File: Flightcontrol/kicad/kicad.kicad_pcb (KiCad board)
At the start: 2 copper layers, 55 x 35.1 mm, 53 parts, among them J1 Conn_01x04_Pin, J2 Conn_01x06, J3 Conn_01x08, J4 Conn_01x01_Pin, J5 Conn_01x05, J6 Conn_01x03_Pin, J7 Conn_01x05, U1 ESP32-S3-WROOM-1U-N16R8, U2 BMP581

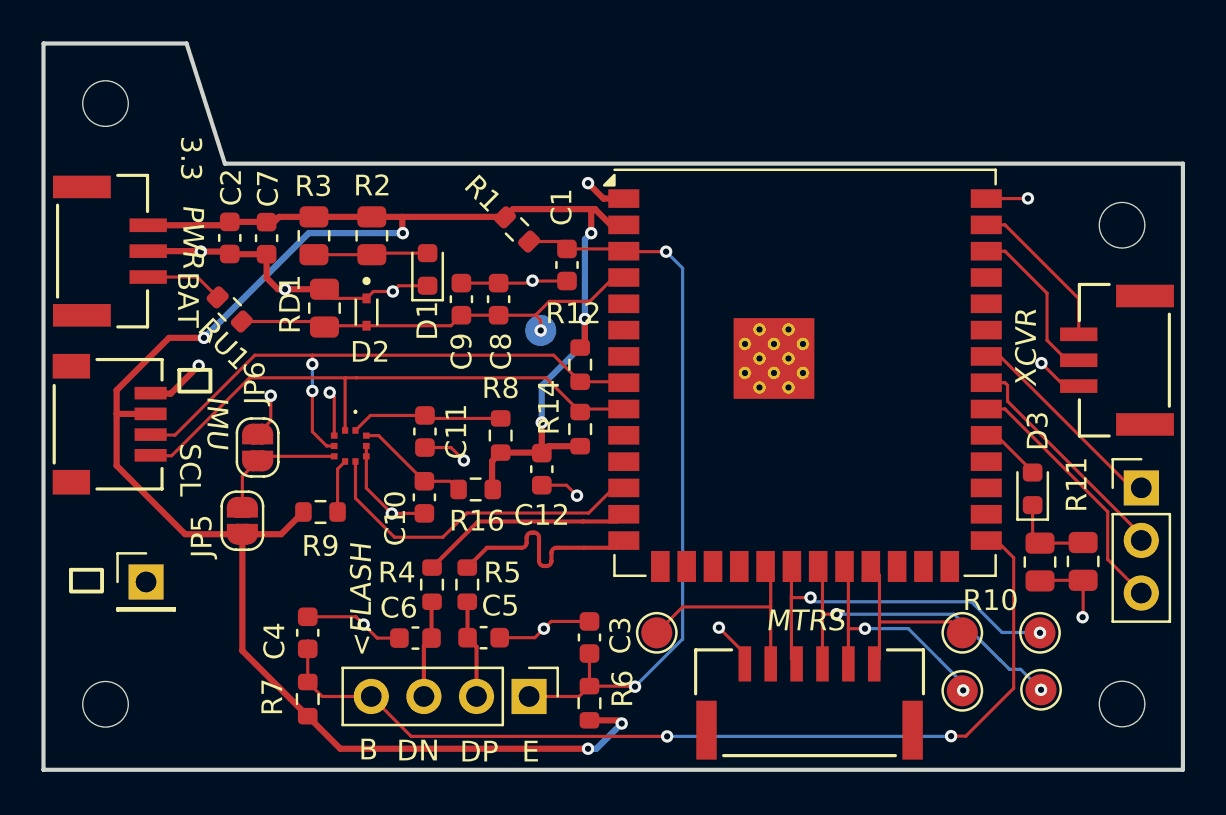
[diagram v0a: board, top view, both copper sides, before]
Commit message: generated pcb files :)
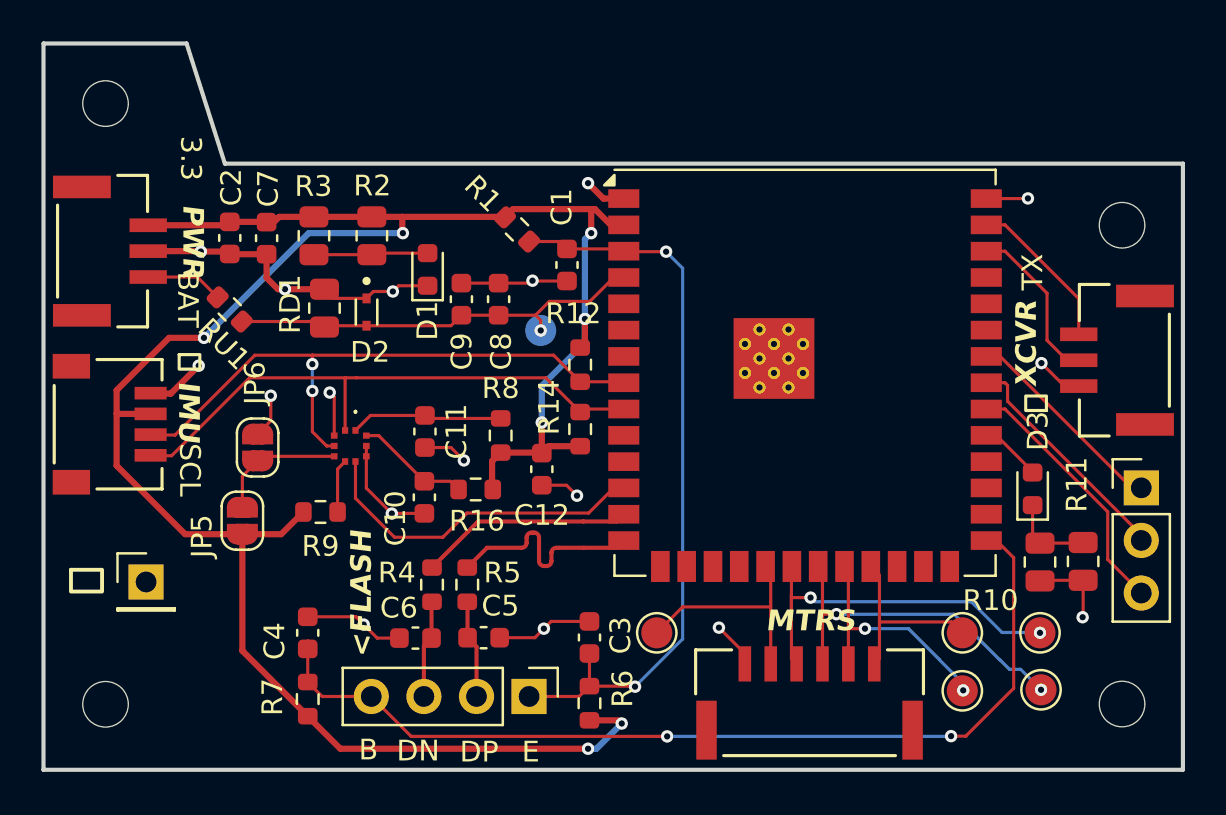
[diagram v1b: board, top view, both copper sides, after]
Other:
- board text added: "TX"
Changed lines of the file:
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@@
 		(embedded_fonts no)
 		(model "BMP581.stp"
+			(hide yes)
 			(offset
 				(xyz 0 0 0)
@@
 		)
 		(embedded_fonts no)
-		(model "${KICAD9_3DMODEL_DIR}/RF_Module.3dshapes/ESP32-S3-WROOM-1U.step"
+		(model "${KIPRJMOD}/dependencies/ESP32_S3_WROOM_1U_N16R8/ESP32-S3-WROOM-1U-N16R8.step"
 			(offset
 				(xyz 0 0 0)
@@
 			)
 			(rotate
-				(xyz 0 0 0)
+				(xyz -90 -0 -0)
 			)
 		)
@@
 		(layer "Edge.Cuts")
 	)
+	(gr_text "TX"
+		(at 176.4792 55.4736 90)
+		(layer "F.SilkS")
+		(effects
+			(font
+				(size 1 1)
+				(thickness 0.15)
+			)
+			(justify left bottom)
+		)
+	)
 	(gr_text "BAT"
 		(at 134.5184 54.5592 270)
@@
 			(font
 				(size 1 1)
-				(thickness 0.15)
+				(thickness 0.2)
+				(bold yes)
 				(italic yes)
 			)
@@
 			(font
 				(size 1 1)
-				(thickness 0.15)
+				(thickness 0.2)
+				(bold yes)
 				(italic yes)
 			)
@@
 			(font
 				(size 1 1)
-				(thickness 0.15)
+				(thickness 0.2)
+				(bold yes)
 				(italic yes)
 			)
@@
 	)
 	(gr_text "⏚"
-		(at 134.5184 59.0804 270)
+		(at 134.5692 58.42 270)
 		(layer "F.SilkS")
 		(effects
 			(font
-				(size 1.5 1.5)
-				(thickness 0.1875)
+				(size 1 1)
+				(thickness 0.15)
 			)
 			(justify left bottom)
@@
 		)
 	)
+	(gr_text "⏚"
+		(at 176.6824 61.4172 90)
+		(layer "F.SilkS")
+		(effects
+			(font
+				(size 1 1)
+				(thickness 0.15)
+			)
+			(justify left bottom)
+		)
+	)
 	(gr_text "MTRS"
 		(at 163 72 0)
@@
 			(font
 				(size 1 1)
-				(thickness 0.15)
+				(thickness 0.2)
+				(bold yes)
 				(italic yes)
 			)
@@
 	)
 	(gr_text "IMU"
-		(at 135.9408 60.5536 270)
+		(at 134.5692 59.8424 270)
 		(layer "F.SilkS")
 		(effects
 			(font
 				(size 1 1)
-				(thickness 0.15)
+				(thickness 0.2)
+				(bold yes)
 				(italic yes)
 			)
@@
 	)
 	(zone
+		(net 0)
+		(net_name "")
+		(layer "F.Mask")
+		(hatch edge 0.5)
+		(connect_pads
+			(clearance 0.5)
+		)
+		(min_thickness 0.25)
+		(filled_areas_thickness no)
+		(fill yes
+			(thermal_gap 0.5)
+			(thermal_bridge_width 0.5)
+		)
+		(polygon
+			(pts
+				(xy 141.986 61.976) (xy 141.986 63.9572) (xy 143.9672 63.9572) (xy 143.9672 61.976) (xy 141.9352 61.976)
+				(xy 141.9352 63.9572) (xy 143.9672 63.9572) (xy 143.9672 61.976)
+			)
+		)
+	)
+	(zone
